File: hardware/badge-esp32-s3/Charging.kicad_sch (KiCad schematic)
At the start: 12 parts, among them P1 PH-2A_C2319, Q3 HL2301A, SW9 SK-12F04-G050, U17 FH2.54-09-02PZD, U4 TP4056

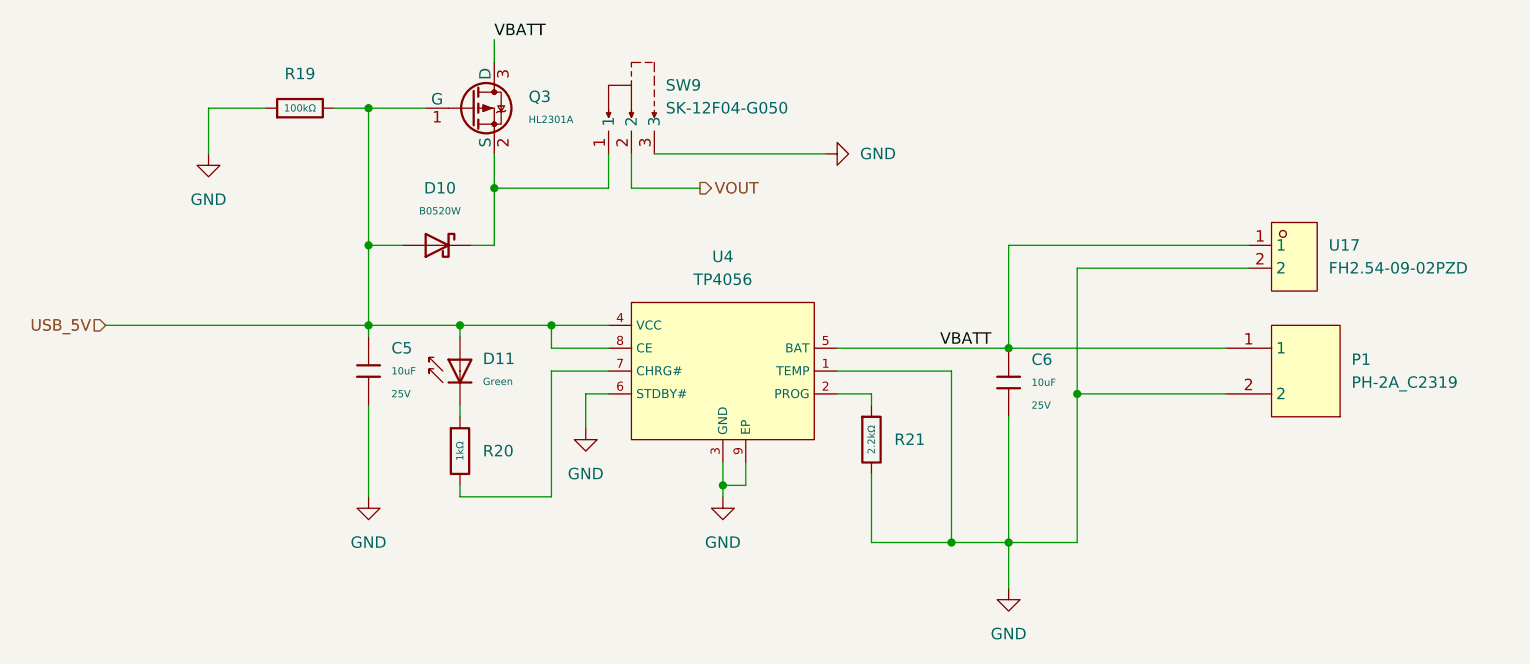
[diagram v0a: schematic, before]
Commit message: Annotate schematic
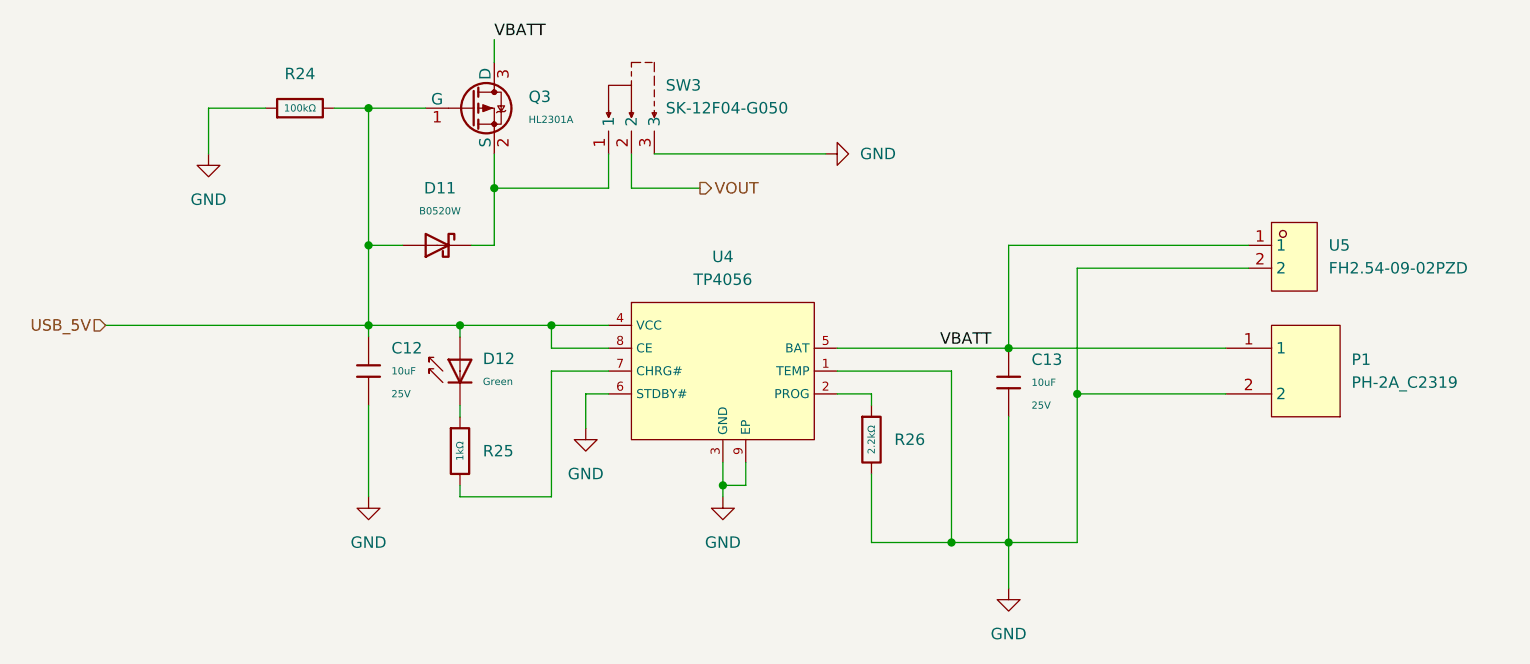
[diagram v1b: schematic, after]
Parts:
- renumbered C5 to C12, C6 to C13, D10 to D11, D11 to D12, R19 to R24, R20 to R25, R21 to R26, SW9 to SW3, U17 to U5
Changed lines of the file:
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@@
 		(dnp no)
 		(fields_autoplaced yes)
-		(property "Reference" "#PWR032"
+		(property "Reference" "#PWR038"
 			(at 146.05 107.95 0)
 			(effects
@@
 			(project ""
 				(path "/e2af9a6c-dbe9-4de2-9ba6-ea213a7300ec/9131a646-b9dc-4004-a7df-1b58b7ca0b9a"
-					(reference "#PWR032")
+					(reference "#PWR038")
 					(unit 1)
 				)
@@
 		(dnp no)
 		(fields_autoplaced yes)
-		(property "Reference" "R20"
+		(property "Reference" "R25"
 			(at 119.38 96.5199 0)
 			(effects
@@
 			(project ""
 				(path "/e2af9a6c-dbe9-4de2-9ba6-ea213a7300ec/9131a646-b9dc-4004-a7df-1b58b7ca0b9a"
-					(reference "R20")
+					(reference "R25")
 					(unit 1)
 				)
@@
 		(dnp no)
 		(fields_autoplaced yes)
-		(property "Reference" "#PWR031"
+		(property "Reference" "#PWR040"
 			(at 177.8 118.11 0)
 			(effects
@@
 			(project ""
 				(path "/e2af9a6c-dbe9-4de2-9ba6-ea213a7300ec/9131a646-b9dc-4004-a7df-1b58b7ca0b9a"
-					(reference "#PWR031")
+					(reference "#PWR040")
 					(unit 1)
 				)
@@
 		(dnp no)
 		(fields_autoplaced yes)
-		(property "Reference" "C6"
+		(property "Reference" "C13"
 			(at 180.34 86.3599 0)
 			(effects
@@
 			(project ""
 				(path "/e2af9a6c-dbe9-4de2-9ba6-ea213a7300ec/9131a646-b9dc-4004-a7df-1b58b7ca0b9a"
-					(reference "C6")
+					(reference "C13")
 					(unit 1)
 				)
@@
 		(dnp no)
 		(fields_autoplaced yes)
-		(property "Reference" "R21"
+		(property "Reference" "R26"
 			(at 165.1 95.2499 0)
 			(effects
@@
 			(project ""
 				(path "/e2af9a6c-dbe9-4de2-9ba6-ea213a7300ec/9131a646-b9dc-4004-a7df-1b58b7ca0b9a"
-					(reference "R21")
+					(reference "R26")
 					(unit 1)
 				)
@@
 		(dnp no)
 		(fields_autoplaced yes)
-		(property "Reference" "#PWR046"
+		(property "Reference" "#PWR039"
 			(at 163.83 63.5 0)
 			(effects
@@
 			(project ""
 				(path "/e2af9a6c-dbe9-4de2-9ba6-ea213a7300ec/9131a646-b9dc-4004-a7df-1b58b7ca0b9a"
-					(reference "#PWR046")
+					(reference "#PWR039")
 					(unit 1)
 				)
@@
 		(dnp no)
 		(fields_autoplaced yes)
-		(property "Reference" "C5"
+		(property "Reference" "C12"
 			(at 109.22 85.0899 0)
 			(effects
@@
 			(project ""
 				(path "/e2af9a6c-dbe9-4de2-9ba6-ea213a7300ec/9131a646-b9dc-4004-a7df-1b58b7ca0b9a"
-					(reference "C5")
+					(reference "C12")
 					(unit 1)
 				)
@@
 		(dnp no)
 		(fields_autoplaced yes)
-		(property "Reference" "#PWR034"
+		(property "Reference" "#PWR037"
 			(at 130.81 100.33 0)
 			(effects
@@
 			(project ""
 				(path "/e2af9a6c-dbe9-4de2-9ba6-ea213a7300ec/9131a646-b9dc-4004-a7df-1b58b7ca0b9a"
-					(reference "#PWR034")
+					(reference "#PWR037")
 					(unit 1)
 				)
@@
 		(dnp no)
 		(fields_autoplaced yes)
-		(property "Reference" "D10"
+		(property "Reference" "D11"
 			(at 114.6175 67.31 90)
 			(effects
@@
 			(project ""
 				(path "/e2af9a6c-dbe9-4de2-9ba6-ea213a7300ec/9131a646-b9dc-4004-a7df-1b58b7ca0b9a"
-					(reference "D10")
+					(reference "D11")
 					(unit 1)
 				)
@@
 		(dnp no)
 		(fields_autoplaced yes)
-		(property "Reference" "R19"
+		(property "Reference" "R24"
 			(at 99.06 54.61 90)
 			(effects
@@
 			(project ""
 				(path "/e2af9a6c-dbe9-4de2-9ba6-ea213a7300ec/9131a646-b9dc-4004-a7df-1b58b7ca0b9a"
-					(reference "R19")
+					(reference "R24")
 					(unit 1)
 				)
@@
 		(dnp no)
 		(fields_autoplaced yes)
-		(property "Reference" "D11"
+		(property "Reference" "D12"
 			(at 119.38 86.2646 0)
 			(effects
@@
 			(project ""
 				(path "/e2af9a6c-dbe9-4de2-9ba6-ea213a7300ec/9131a646-b9dc-4004-a7df-1b58b7ca0b9a"
-					(reference "D11")
+					(reference "D12")
 					(unit 1)
 				)
@@
 		(dnp no)
 		(fields_autoplaced yes)
-		(property "Reference" "#PWR033"
+		(property "Reference" "#PWR035"
 			(at 88.9 69.85 0)
 			(effects
@@
 			(project ""
 				(path "/e2af9a6c-dbe9-4de2-9ba6-ea213a7300ec/9131a646-b9dc-4004-a7df-1b58b7ca0b9a"
-					(reference "#PWR033")
+					(reference "#PWR035")
 					(unit 1)
 				)
@@
 		(dnp no)
 		(fields_autoplaced yes)
-		(property "Reference" "SW9"
+		(property "Reference" "SW3"
 			(at 139.7 55.8799 0)
 			(effects
@@
 			(project "badge-esp32-s3"
 				(path "/e2af9a6c-dbe9-4de2-9ba6-ea213a7300ec/9131a646-b9dc-4004-a7df-1b58b7ca0b9a"
-					(reference "SW9")
+					(reference "SW3")
 					(unit 1)
 				)
@@
 		(dnp no)
 		(fields_autoplaced yes)
-		(property "Reference" "U17"
+		(property "Reference" "U5"
 			(at 213.36 73.6599 0)
 			(effects
@@
 			(project ""
 				(path "/e2af9a6c-dbe9-4de2-9ba6-ea213a7300ec/9131a646-b9dc-4004-a7df-1b58b7ca0b9a"
-					(reference "U17")
+					(reference "U5")
 					(unit 1)
 				)

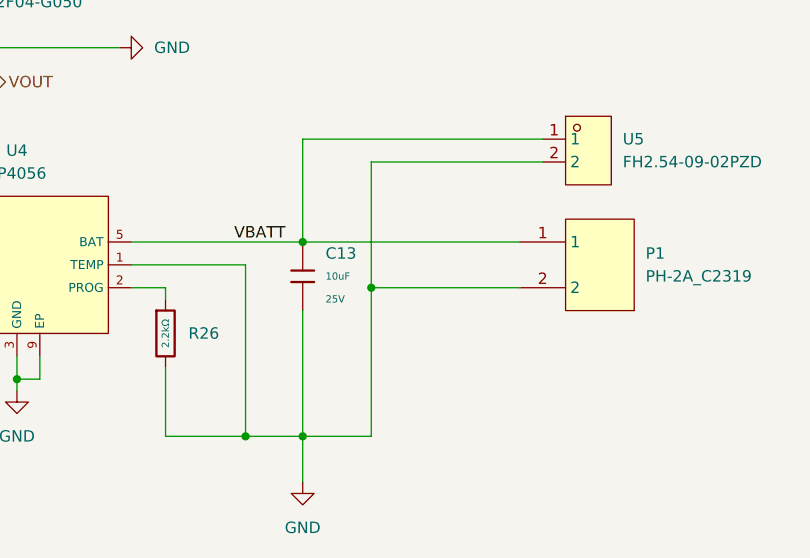
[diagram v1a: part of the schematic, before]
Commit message: schematic_pwr
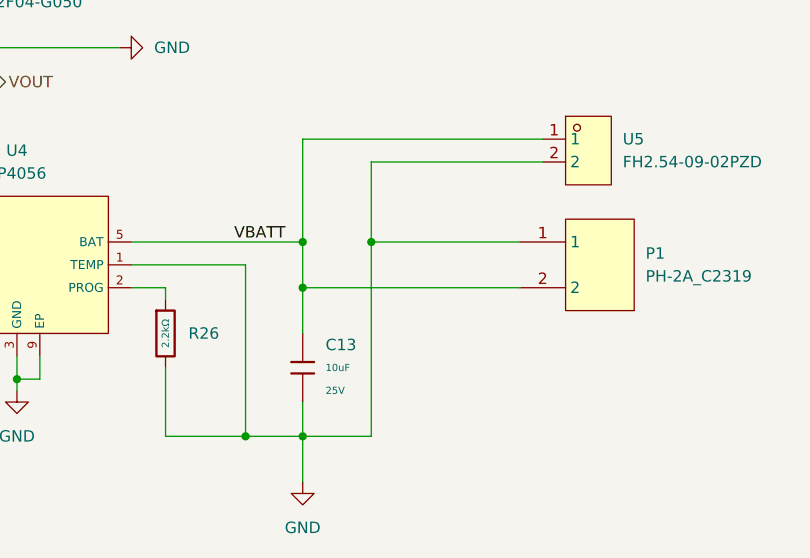
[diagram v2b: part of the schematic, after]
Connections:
- net GND: now also P1.1; no longer P1.2
- net VBATT: now also P1.2; no longer P1.1
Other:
- moved on the sheet: C13
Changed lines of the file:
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@@
+	)
+	(junction
+		(at 177.8 90.17)
+		(diameter 0)
+		(color 0 0 0 0)
 	)
 	(junction
@@
 	)
 	(junction
+		(at 185.42 85.09)
+		(diameter 0)
+		(color 0 0 0 0)
+	)
+	(junction
 		(at 120.65 67.31)
 		(diameter 0)
@@
 	)
 	(junction
-		(at 185.42 90.17)
-		(diameter 0)
-		(color 0 0 0 0)
-	)
-	(junction
 		(at 106.68 73.66)
 		(diameter 0)
@@
 	(wire
 		(pts
-			(xy 185.42 76.2) (xy 185.42 90.17)
-		)
-		(stroke
-			(width 0)
-			(type default)
-		)
-	)
-	(wire
-		(pts
 			(xy 118.11 73.66) (xy 120.65 73.66)
 		)
@@
 	(wire
 		(pts
-			(xy 185.42 90.17) (xy 201.93 90.17)
-		)
-		(stroke
-			(width 0)
-			(type default)
-		)
-	)
-	(wire
-		(pts
 			(xy 185.42 106.68) (xy 177.8 106.68)
 		)
@@
 	(wire
 		(pts
+			(xy 177.8 95.25) (xy 177.8 90.17)
+		)
+		(stroke
+			(width 0)
+			(type default)
+		)
+	)
+	(wire
+		(pts
 			(xy 130.81 90.17) (xy 133.35 90.17)
 		)
@@
 	(wire
 		(pts
-			(xy 177.8 85.09) (xy 201.93 85.09)
-		)
-		(stroke
-			(width 0)
-			(type default)
-		)
-	)
-	(wire
-		(pts
 			(xy 88.9 58.42) (xy 88.9 63.5)
 		)
@@
 	(wire
 		(pts
+			(xy 177.8 90.17) (xy 201.93 90.17)
+		)
+		(stroke
+			(width 0)
+			(type default)
+		)
+	)
+	(wire
+		(pts
+			(xy 185.42 85.09) (xy 201.93 85.09)
+		)
+		(stroke
+			(width 0)
+			(type default)
+		)
+	)
+	(wire
+		(pts
 			(xy 106.68 91.44) (xy 106.68 101.6)
 		)
@@
 	(wire
 		(pts
+			(xy 177.8 90.17) (xy 177.8 85.09)
+		)
+		(stroke
+			(width 0)
+			(type default)
+		)
+	)
+	(wire
+		(pts
 			(xy 116.84 100.33) (xy 116.84 101.6)
 		)
@@
 	(wire
 		(pts
-			(xy 185.42 90.17) (xy 185.42 106.68)
-		)
-		(stroke
-			(width 0)
-			(type default)
-		)
-	)
-	(wire
-		(pts
-			(xy 177.8 92.71) (xy 177.8 106.68)
+			(xy 185.42 76.2) (xy 185.42 85.09)
+		)
+		(stroke
+			(width 0)
+			(type default)
+		)
+	)
+	(wire
+		(pts
+			(xy 177.8 102.87) (xy 177.8 106.68)
 		)
 		(stroke
@@
 		(pts
 			(xy 110.49 73.66) (xy 106.68 73.66)
+		)
+		(stroke
+			(width 0)
+			(type default)
+		)
+	)
+	(wire
+		(pts
+			(xy 185.42 85.09) (xy 185.42 106.68)
 		)
 		(stroke
@@
 	(symbol
 		(lib_id "PCM_JLCPCB-Capacitors:0603,10uF,(2)")
-		(at 177.8 88.9 0)
+		(at 177.8 99.06 0)
 		(unit 1)
 		(exclude_from_sim no)
@@
 		(fields_autoplaced yes)
 		(property "Reference" "C13"
-			(at 180.34 86.3599 0)
+			(at 180.34 96.5199 0)
 			(effects
 				(font
@@
 		)
 		(property "Value" "10uF"
-			(at 180.34 88.9 0)
+			(at 180.34 99.06 0)
 			(effects
 				(font
@@
 		)
 		(property "Footprint" "PCM_JLCPCB:C_0603"
-			(at 176.022 88.9 90)
+			(at 176.022 99.06 90)
 			(effects
 				(font
@@
 		)
 		(property "Datasheet" "https://www.lcsc.com/datasheet/lcsc_datasheet_2304140030_Samsung-Electro-Mechanics-CL10A106MA8NRNC_C96446.pdf"
-			(at 177.8 88.9 0)
+			(at 177.8 99.06 0)
 			(effects
 				(font
@@
 		)
 		(property "Description" "25V 10uF X5R ±20% 0603 Multilayer Ceramic Capacitors MLCC - SMD/SMT ROHS"
-			(at 177.8 88.9 0)
+			(at 177.8 99.06 0)
 			(effects
 				(font
@@
 		)
 		(property "LCSC" "C96446"
-			(at 177.8 88.9 0)
+			(at 177.8 99.06 0)
 			(effects
 				(font
@@
 		)
 		(property "Stock" "2627344"
-			(at 177.8 88.9 0)
+			(at 177.8 99.06 0)
 			(effects
 				(font
@@
 		)
 		(property "Price" "0.021USD"
-			(at 177.8 88.9 0)
+			(at 177.8 99.06 0)
 			(effects
 				(font
@@
 		)
 		(property "Process" "SMT"
-			(at 177.8 88.9 0)
+			(at 177.8 99.06 0)
 			(effects
 				(font
@@
 		)
 		(property "Minimum Qty" "20"
-			(at 177.8 88.9 0)
+			(at 177.8 99.06 0)
 			(effects
 				(font
@@
 		)
 		(property "Attrition Qty" "8"
-			(at 177.8 88.9 0)
+			(at 177.8 99.06 0)
 			(effects
 				(font
@@
 		)
 		(property "Class" "Basic Component"
-			(at 177.8 88.9 0)
+			(at 177.8 99.06 0)
 			(effects
 				(font
@@
 		)
 		(property "Category" "Capacitors,Multilayer Ceramic Capacitors MLCC - SMD/SMT"
-			(at 177.8 88.9 0)
+			(at 177.8 99.06 0)
 			(effects
 				(font
@@
 		)
 		(property "Manufacturer" "Samsung Electro-Mechanics"
-			(at 177.8 88.9 0)
+			(at 177.8 99.06 0)
 			(effects
 				(font
@@
 		)
 		(property "Part" "CL10A106MA8NRNC"
-			(at 177.8 88.9 0)
+			(at 177.8 99.06 0)
 			(effects
 				(font
@@
 		)
 		(property "Voltage Rated" "25V"
-			(at 180.34 91.44 0)
+			(at 180.34 101.6 0)
 			(effects
 				(font
@@
 		)
 		(property "Tolerance" "±20%"
-			(at 177.8 88.9 0)
+			(at 177.8 99.06 0)
 			(effects
 				(font
@@
 		)
 		(property "Capacitance" "10uF"
-			(at 177.8 88.9 0)
+			(at 177.8 99.06 0)
 			(effects
 				(font
@@
 		)
 		(property "Temperature Coefficient" "X5R"
-			(at 177.8 88.9 0)
-			(effects
-				(font
+			(at 177.8 99.06 0)
+			(effects
+				(font
